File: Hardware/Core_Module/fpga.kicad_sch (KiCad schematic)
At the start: 26 parts, among them U101 TPS7A20L_1V2, U102 ICE40UL1K-CM36AI, U103 TPS7A20L_2V5, U104 TPS7A20L_3V3, U105 N25Q032A, Y101 12MHz

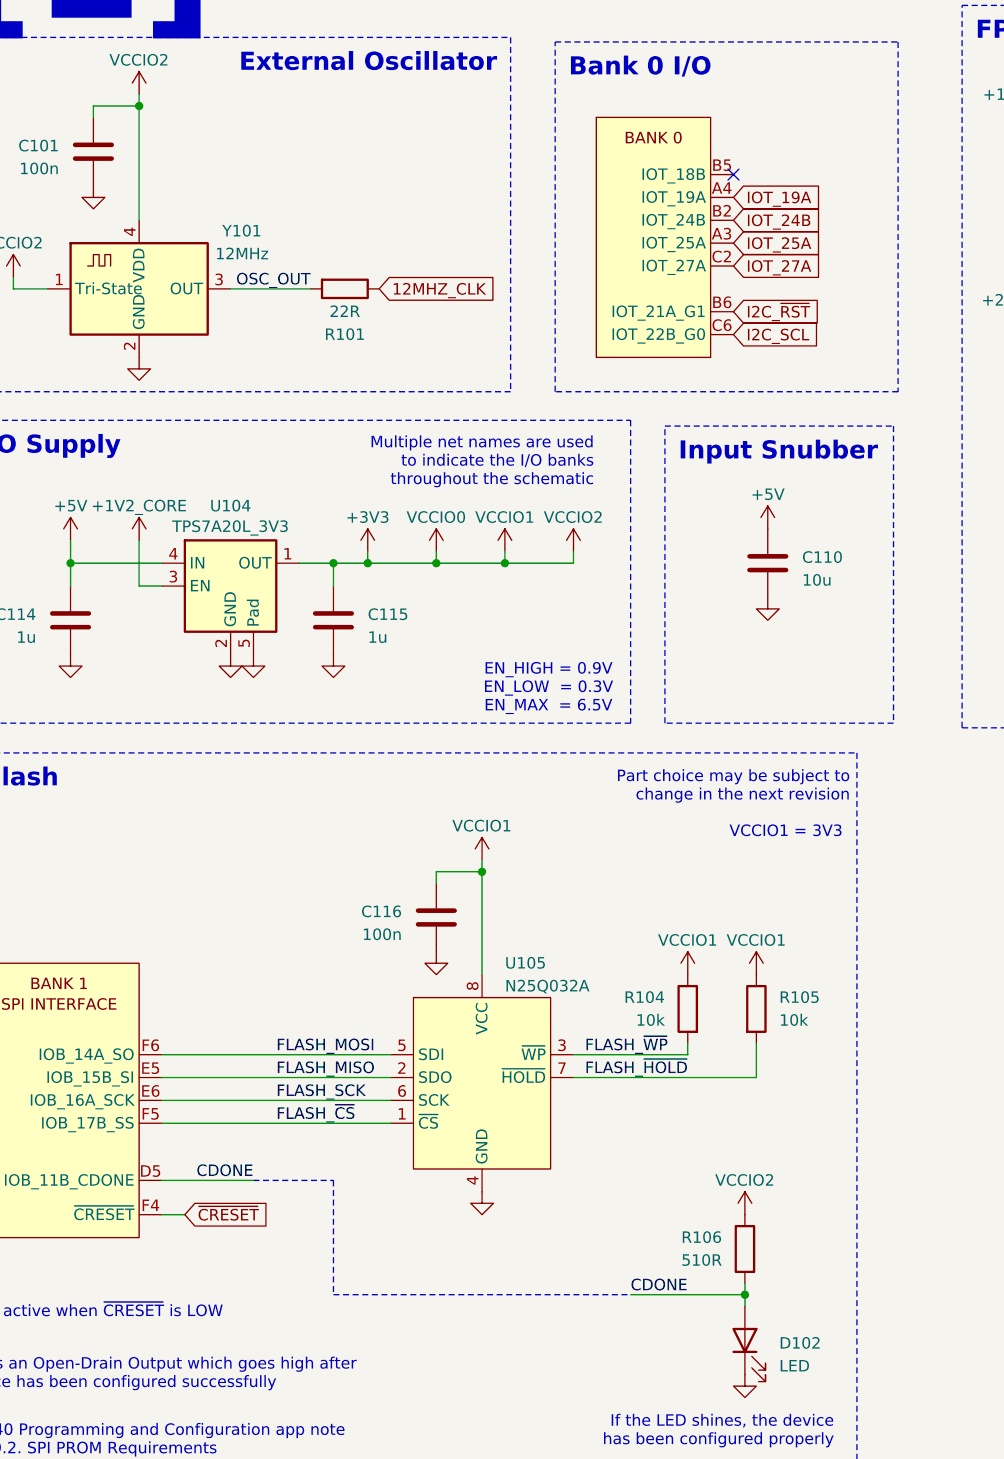
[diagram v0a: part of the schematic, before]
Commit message: Finished Lattice Core, waiting for PCB Review
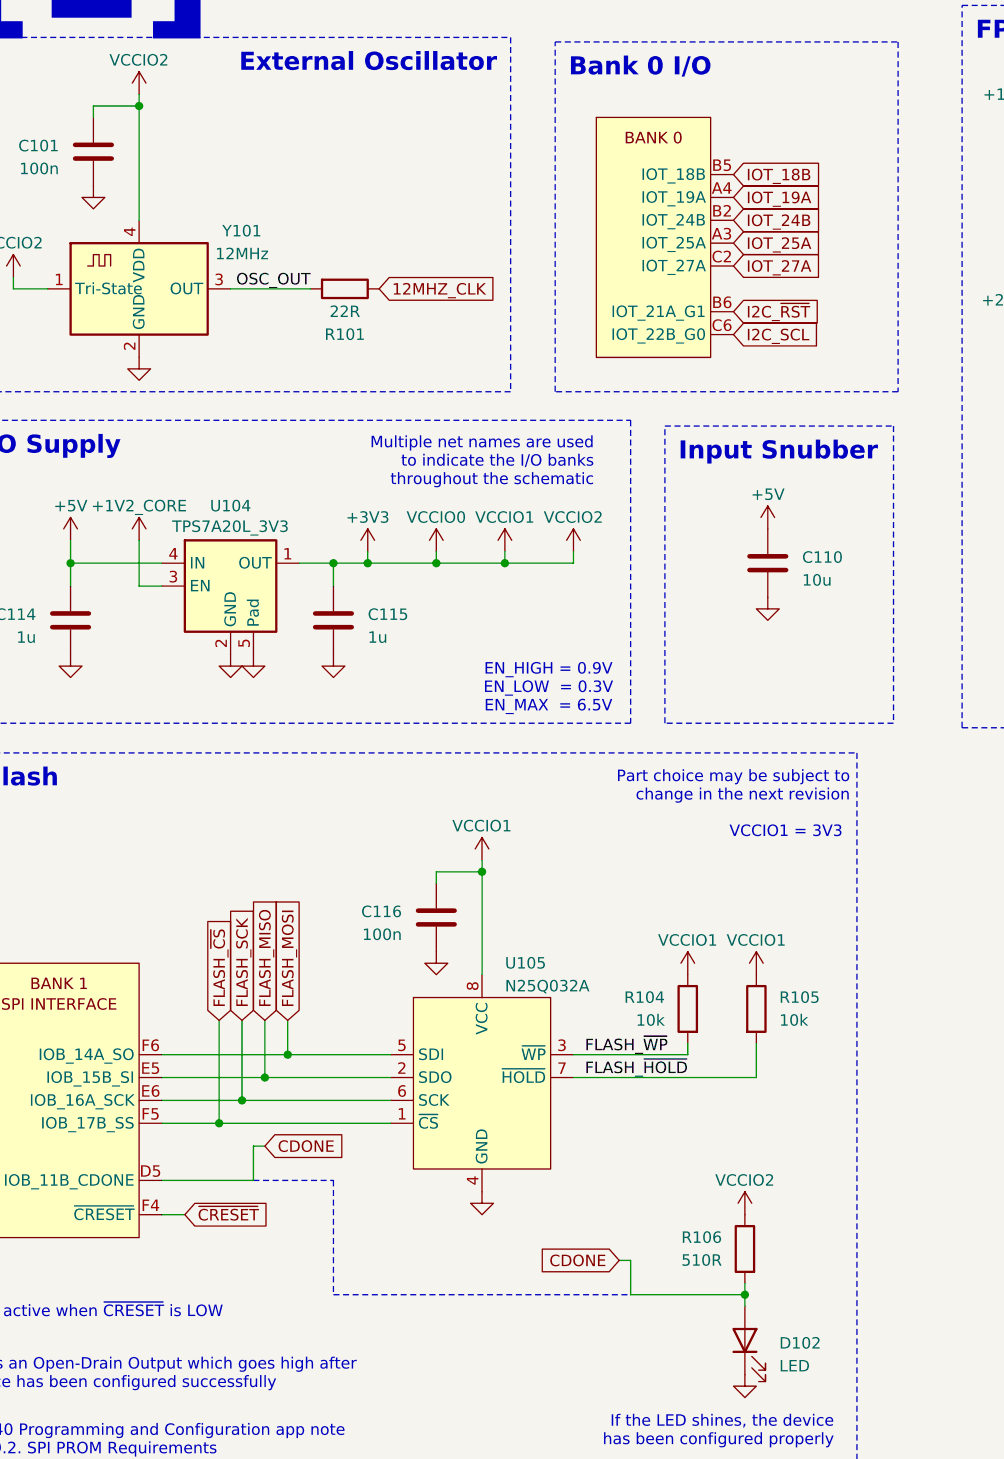
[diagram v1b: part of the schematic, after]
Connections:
- net IOT_18B: now reaches U102.B5 (IOT_18B)
- no-connect marks 1 -> 0

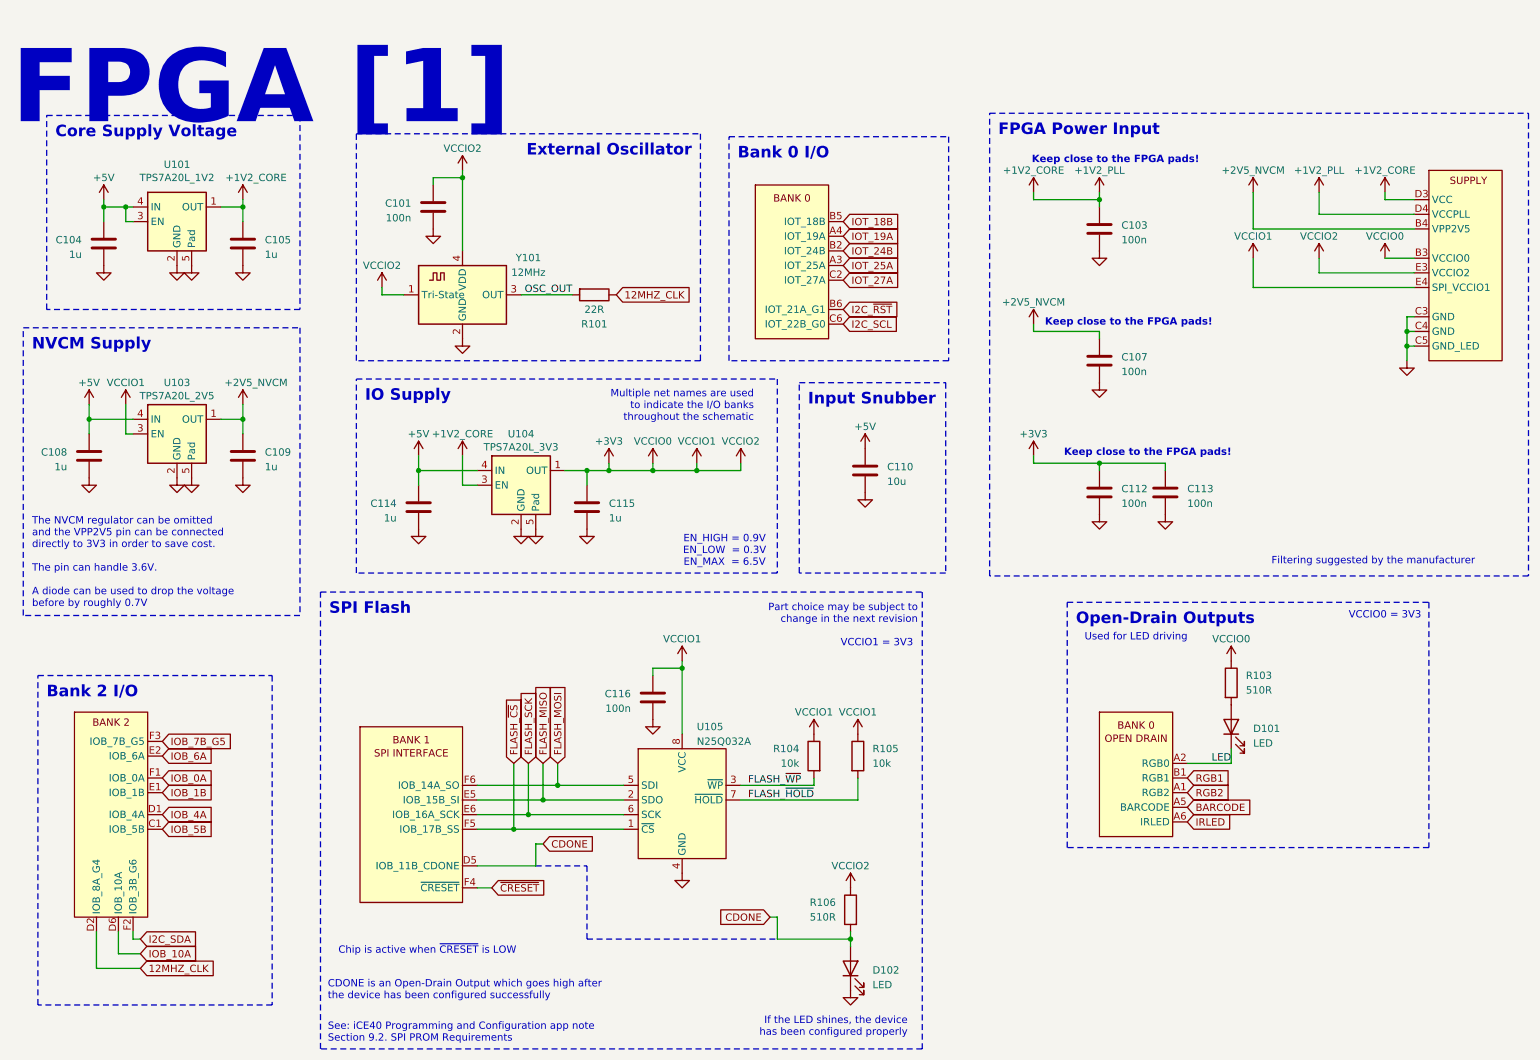
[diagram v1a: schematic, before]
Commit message: Advanced Intel Core Module Development
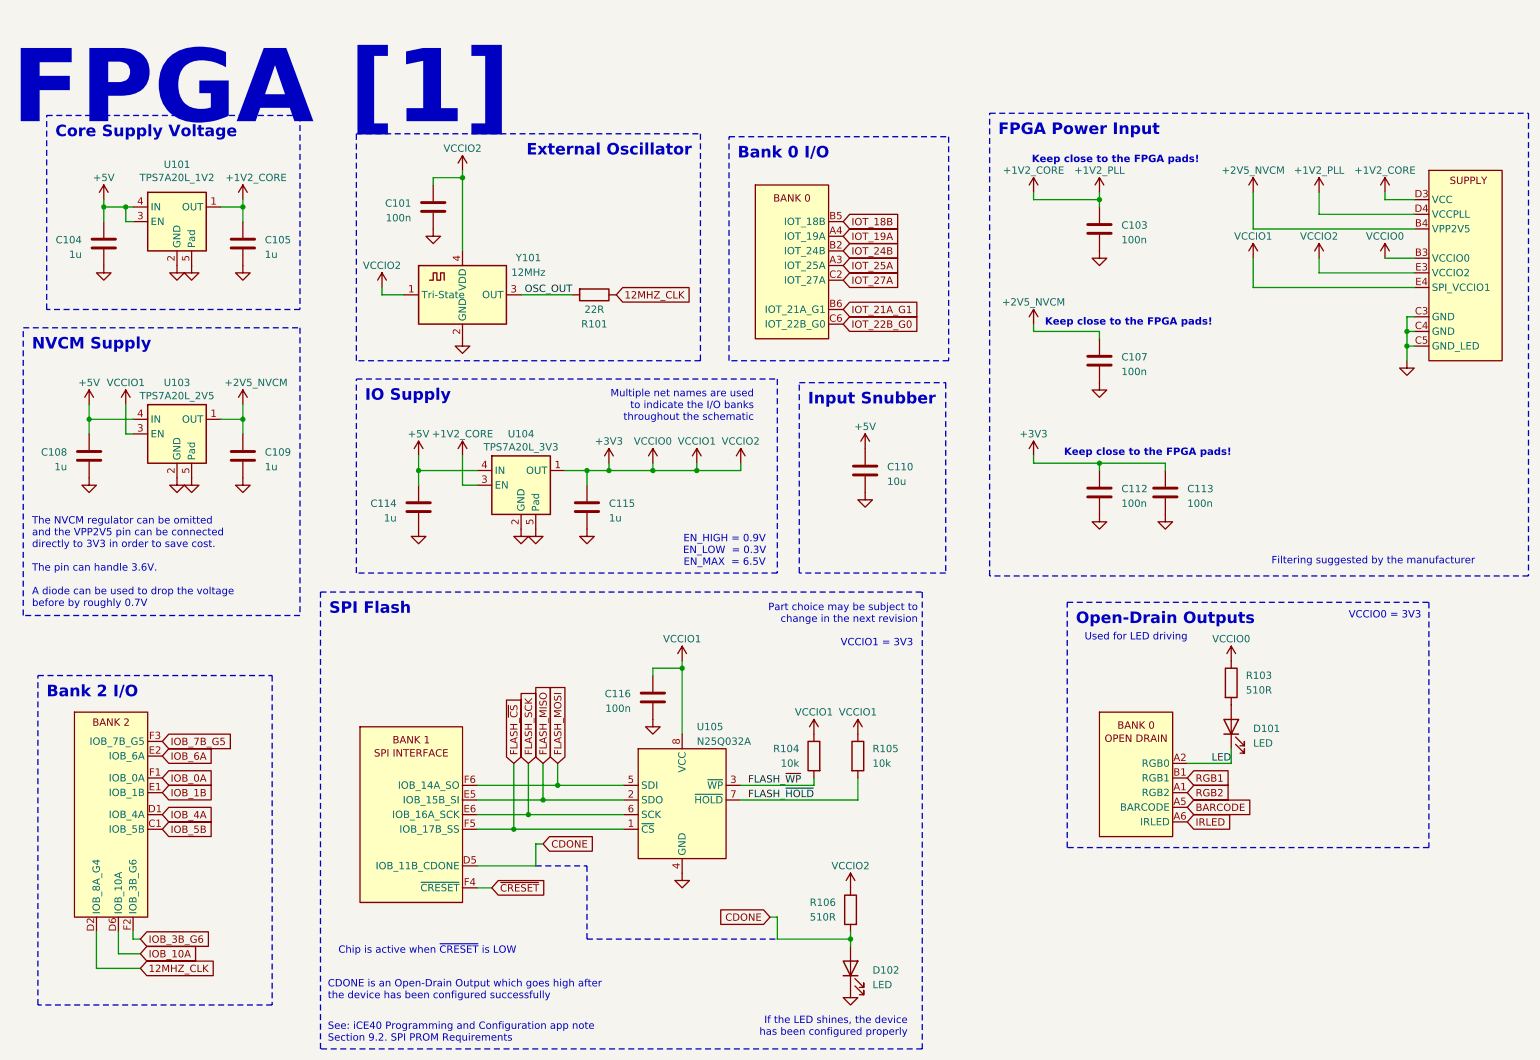
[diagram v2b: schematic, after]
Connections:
- net I2C_SCL renamed IOT_22B_G0
- net I2C_SDA renamed IOB_3B_G6
- net I2C_~{RST} renamed IOT_21A_G1
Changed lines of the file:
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@@
 		)
 	)
-	(global_label "I2C_~{RST}"
+	(global_label "IOT_21A_G1"
 		(shape input)
 		(at 160.02 66.04 0)
@@
 		)
 		(property "Intersheetrefs" "${INTERSHEET_REFS}"
-			(at 170.5042 66.04 0)
+			(at 173.8304 66.04 0)
 			(hide yes)
 			(show_name no)
@@
 		)
 	)
-	(global_label "I2C_SDA"
+	(global_label "IOB_3B_G6"
 		(shape input)
 		(at 38.1 175.26 0)
@@
 		)
 		(property "Intersheetrefs" "${INTERSHEET_REFS}"
-			(at 48.7052 175.26 0)
+			(at 51.1847 175.26 0)
 			(hide yes)
 			(show_name no)
@@
 		)
 	)
-	(global_label "I2C_SCL"
+	(global_label "IOT_22B_G0"
 		(shape input)
 		(at 160.02 68.58 0)
@@
 		)
 		(property "Intersheetrefs" "${INTERSHEET_REFS}"
-			(at 170.5647 68.58 0)
-			(hide yes)
-			(show_name no)
+			(at 174.0118 68.58 0)
+			(hide yes)
+			(show_name no)
